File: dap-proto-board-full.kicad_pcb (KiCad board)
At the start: 6 copper layers, 42.2 x 61.4 mm, 102 parts, among them J1 SFV18R-1STE1HLF, J2 UJ20-C-H-G-SMT-1-P16-TR, J3 SJ-3523-SMT, J4 JST_SH_SM03B-SRSS-TB, J5 JST_PH_S2B-PH-SM4, J6 Conn_01x06, J7 Conn_01x08, SW1 B3U-1000P, SW2 B3U-1000P, U1 TPD1E05U06DPY, U10 nPM1300-QEXX, U11 TPS22917DBV, U12 TPS63031DSK, U2 TAD5212, U3 TXS0108ERGYR, U4 W25Q64JWUUIQ, U5 TXS0108ERGYR, U6 MSD-11-A, U7 APS6404L-SQRH-ZR, U8 RP2350A, U9 TLV73311PDBV, Y1 SIT8021AI-J4-XXS-12.288E, Y2 SIT8021AI-J4-XXS-11.289E, Y3 ABM8-272-T3

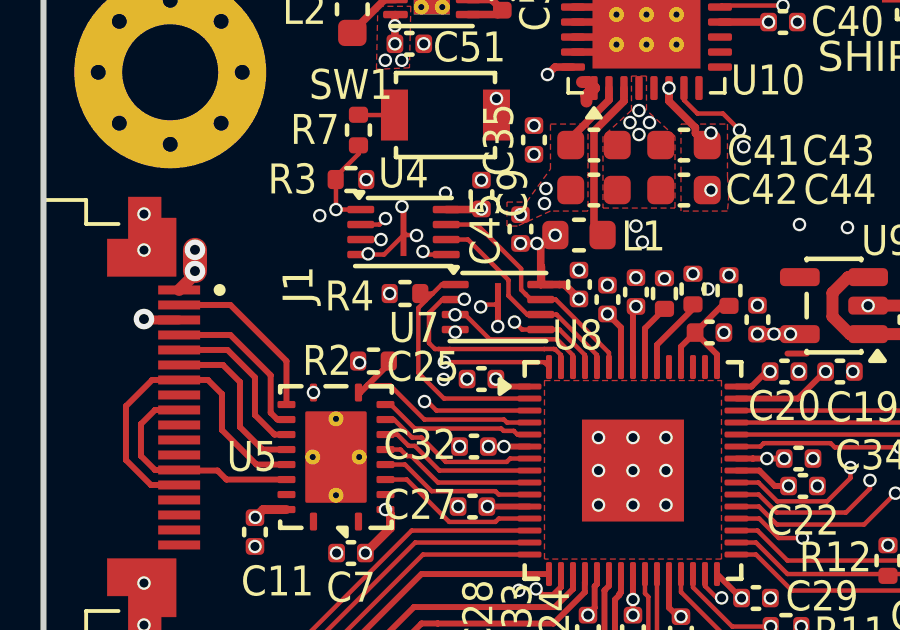
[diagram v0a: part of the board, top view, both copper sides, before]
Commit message: I forgort what I did
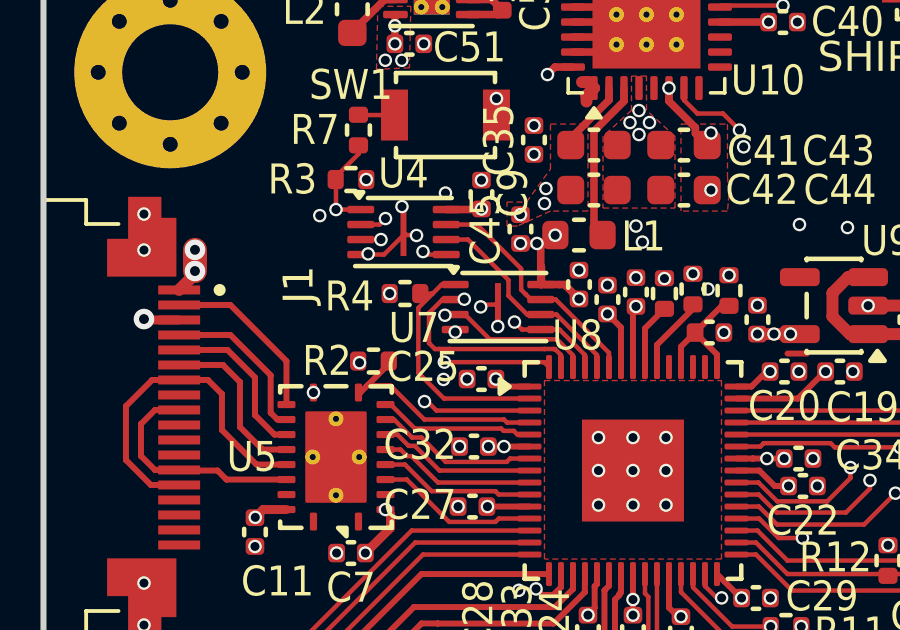
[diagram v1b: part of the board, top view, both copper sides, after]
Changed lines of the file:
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@@
+	)
+	(segment
+		(start 110.4 81.408102)
+		(end 110.4 81.8)
+		(width 0.150114)
+		(layer "F.Cu")
+		(net "/QSPI_SD2")
+	)
+	(segment
+		(start 109.868955 80.877057)
+		(end 110.4 81.408102)
+		(width 0.150114)
+		(layer "F.Cu")
+		(net "/QSPI_SD2")
 	)
 	(segment
@@
 	)
 	(segment
-		(start 109.868955 80.877057)
-		(end 110.4 81.408102)
-		(width 0.150114)
-		(layer "F.Cu")
-		(net "/QSPI_SD2")
-	)
-	(segment
-		(start 106.470716 80.05722)
-		(end 106.486498 80.073002)
-		(width 0.150114)
-		(layer "F.Cu")
-		(net "/QSPI_SD2")
-	)
-	(segment
-		(start 106.451998 80.073002)
-		(end 106.475 80.05)
+		(start 106.486498 80.073002)
+		(end 106.823874 80.073002)
 		(width 0.150114)
 		(layer "F.Cu")
@@
 	)
 	(segment
-		(start 106.486498 80.073002)
-		(end 106.823874 80.073002)
+		(start 106.486497 80.073001)
+		(end 106.486498 80.073002)
 		(width 0.150114)
 		(layer "F.Cu")
@@
 	)
 	(segment
-		(start 110.4 81.408102)
-		(end 110.4 81.8)
+		(start 106.130949 80.073001)
+		(end 106.486497 80.073001)
+		(width 0.150114)
+		(layer "F.Cu")
+		(net "/QSPI_SD2")
+	)
+	(segment
+		(start 106.451998 80.073002)
+		(end 106.475 80.05)
 		(width 0.150114)
 		(layer "F.Cu")
@@
 	)
 	(via
-		(at 106.470716 80.05722)
+		(at 106.130949 80.073001)
 		(size 0.45)
 		(drill 0.3)
@@
 	)
 	(segment
-		(start 105.973002 80.073002)
-		(end 104 78.1)
+		(start 104 78.1)
+		(end 104 77.55)
 		(width 0.150114)
 		(layer "In2.Cu")
@@
 	)
 	(segment
-		(start 106.470716 80.05722)
-		(end 106.454934 80.073002)
-		(width 0.150114)
-		(layer "In2.Cu")
-		(net "/QSPI_SD2")
-	)
-	(segment
-		(start 106.454934 80.073002)
+		(start 106.130948 80.073002)
 		(end 105.973002 80.073002)
 		(width 0.150114)
@@
 	)
 	(segment
-		(start 104 78.1)
-		(end 104 77.55)
+		(start 106.130949 80.073001)
+		(end 106.130948 80.073002)
 		(width 0.150114)
 		(layer "In2.Cu")
+		(net "/QSPI_SD2")
+	)
+	(segment
+		(start 105.973002 80.073002)
+		(end 104 78.1)
+		(width 0.150114)
+		(layer "In2.Cu")
